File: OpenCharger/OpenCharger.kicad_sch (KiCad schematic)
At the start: 3 parts, among them J1 Conn_01x02, J2 Conn_01x03, J3 Conn_01x02

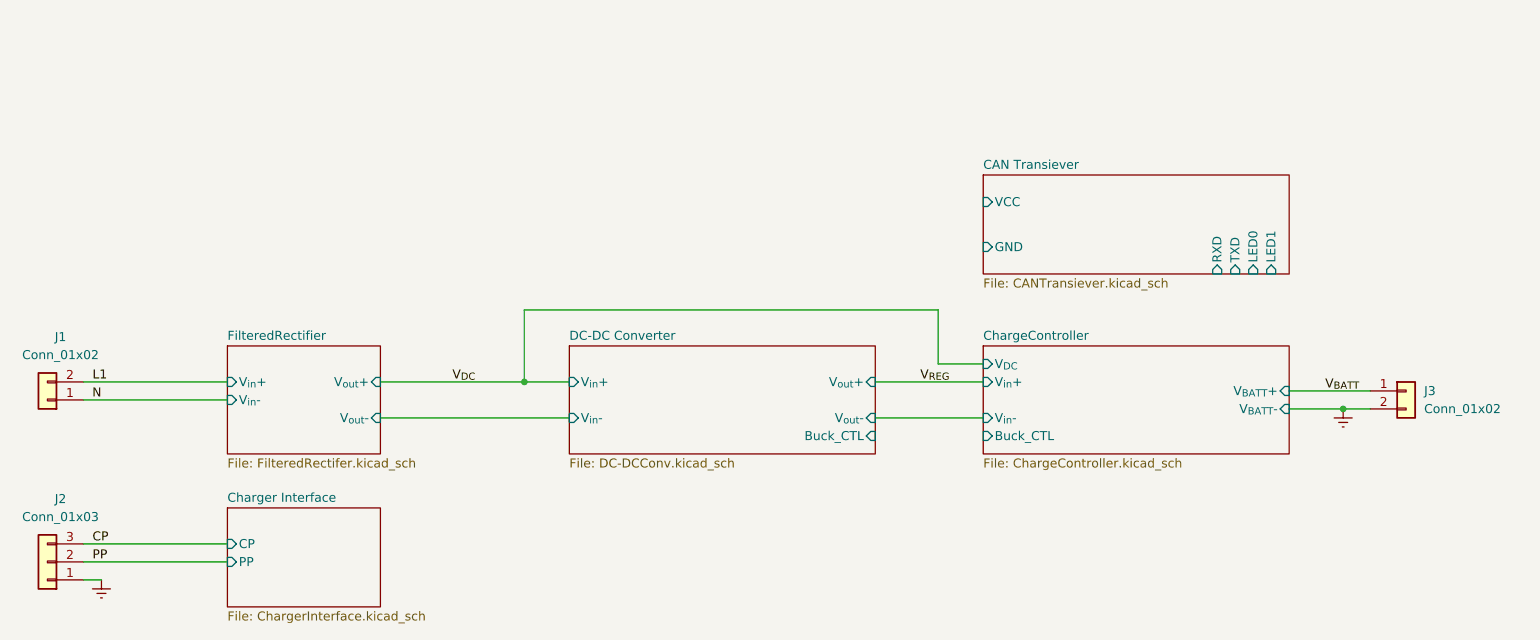
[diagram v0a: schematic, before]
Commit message: updated
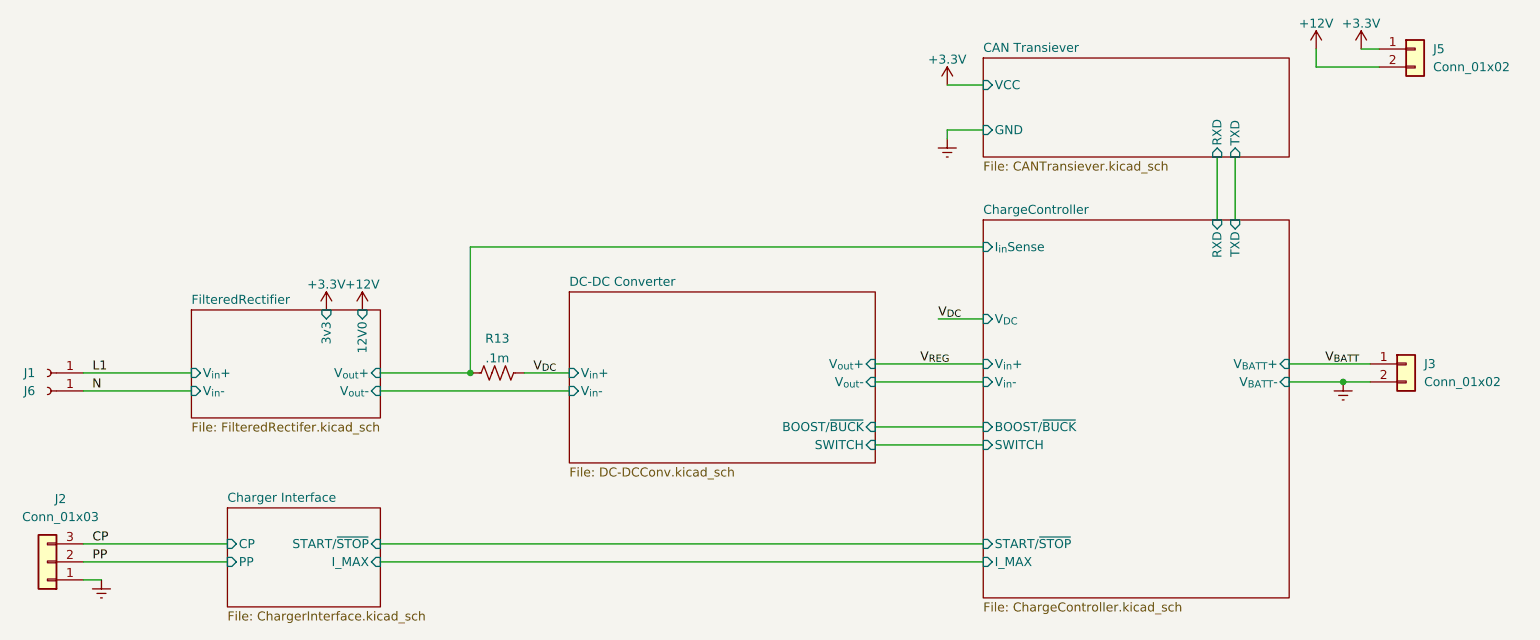
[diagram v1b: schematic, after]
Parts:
- removed J1: Conn_01x02, Connector:Banana_Jack_2Pin, symbol Connector_Generic:Conn_01x02
- added J1, J6: Conn_01x01_Female, Connector:Banana_Jack_1Pin, symbol Connector:Conn_01x01_Female
- added J5: Conn_01x02, Connector_PinHeader_2.54mm:PinHeader_1x02_P2.54mm_Vertical, symbol Connector_Generic:Conn_01x02
- added R13: .1m, symbol Device:R_US
- J2: footprint Connector:Banana_Jack_3Pin -> Connector_PinHeader_2.54mm:PinHeader_1x03_P2.54mm_Vertical
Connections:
- net L1: now also J1.1 (Pin_1)
- net N: now also J6.1 (Pin_1)
- net V_{DC}: now also R13.2
- new net +12V: J5.2 (Pin_2)
- new net +3V3: J5.1 (Pin_1)
- new net ChargeController/I_{in}Sense: R13.1
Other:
- sheet CAN Transiever ports: added none; removed LED0, LED1
- sheet ChargeController ports: added BOOST/~{BUCK}, I_MAX, I_{in}Sense, RXD, START/~{STOP}, SWITCH, TXD; removed Buck_CTL
- sheet Charger Interface ports: added I_MAX, START/~{STOP}; removed none
- sheet DC-DC Converter ports: added BOOST/~{BUCK}, SWITCH; removed Buck_CTL
- sheet FilteredRectifier ports: added 12V0, 3v3; removed none
- moved on the sheet: J3
